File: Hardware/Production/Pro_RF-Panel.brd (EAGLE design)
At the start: 101.9 x 104.9 mm, 612 parts, among them U1 MCP73831, U10 915MHz, U11 ATMEGA32U4, U12 MIC5219-3.3, U13 MCP73831, U14 915MHz, U15 ATMEGA32U4, U16 MIC5219-3.3, U17 MCP73831, U18 915MHz, U19 ATMEGA32U4, U2 915MHz, U20 MIC5219-3.3, U21 MCP73831, U22 915MHz, U23 ATMEGA32U4, U24 MIC5219-3.3, U3 MCP73831, U4 915MHz, U5 ATMEGA32U4, U6 MIC5219-3.3, U7 ATMEGA32U4, U8 MIC5219-3.3, U9 MCP73831, Y1 8MHz, Y2 8MHz, Y3 8MHz, Y4 8MHz, Y5 8MHz, Y6 8MHz

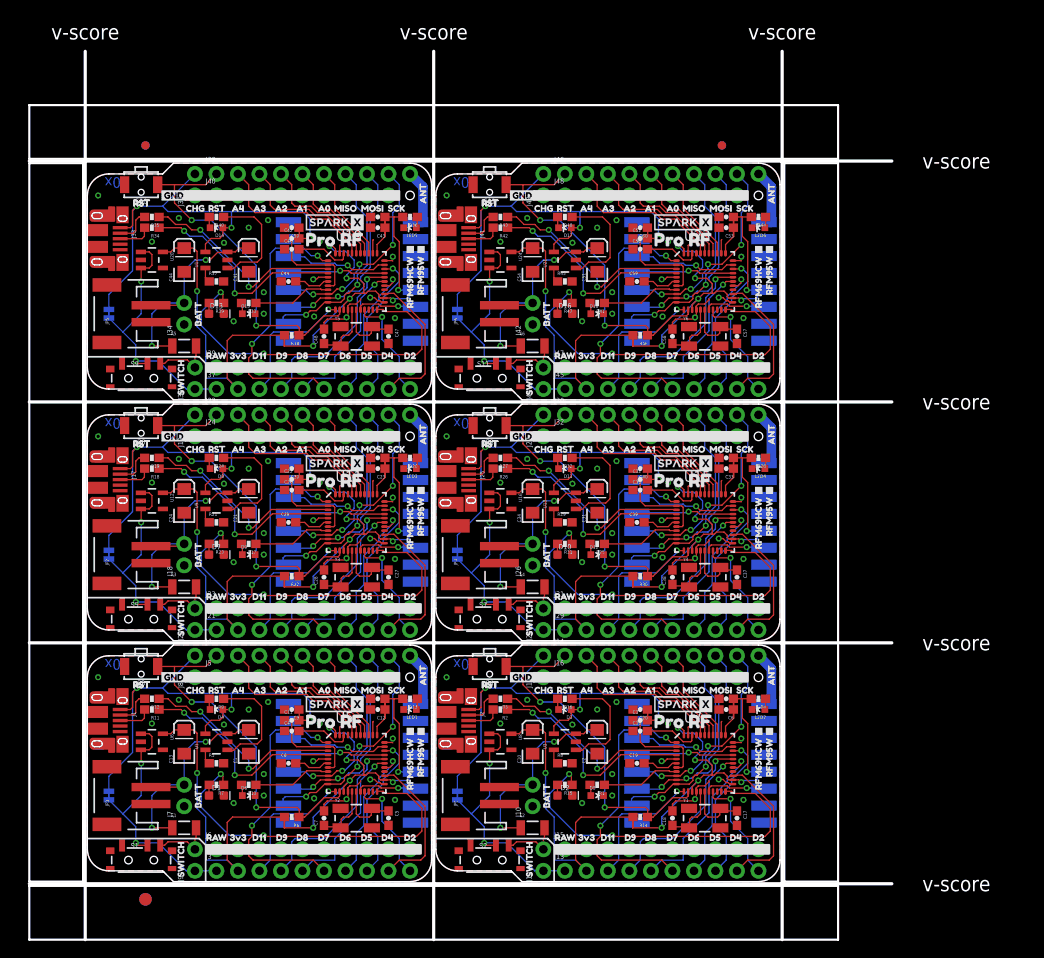
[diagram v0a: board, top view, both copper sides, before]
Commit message: Many updates. v02.
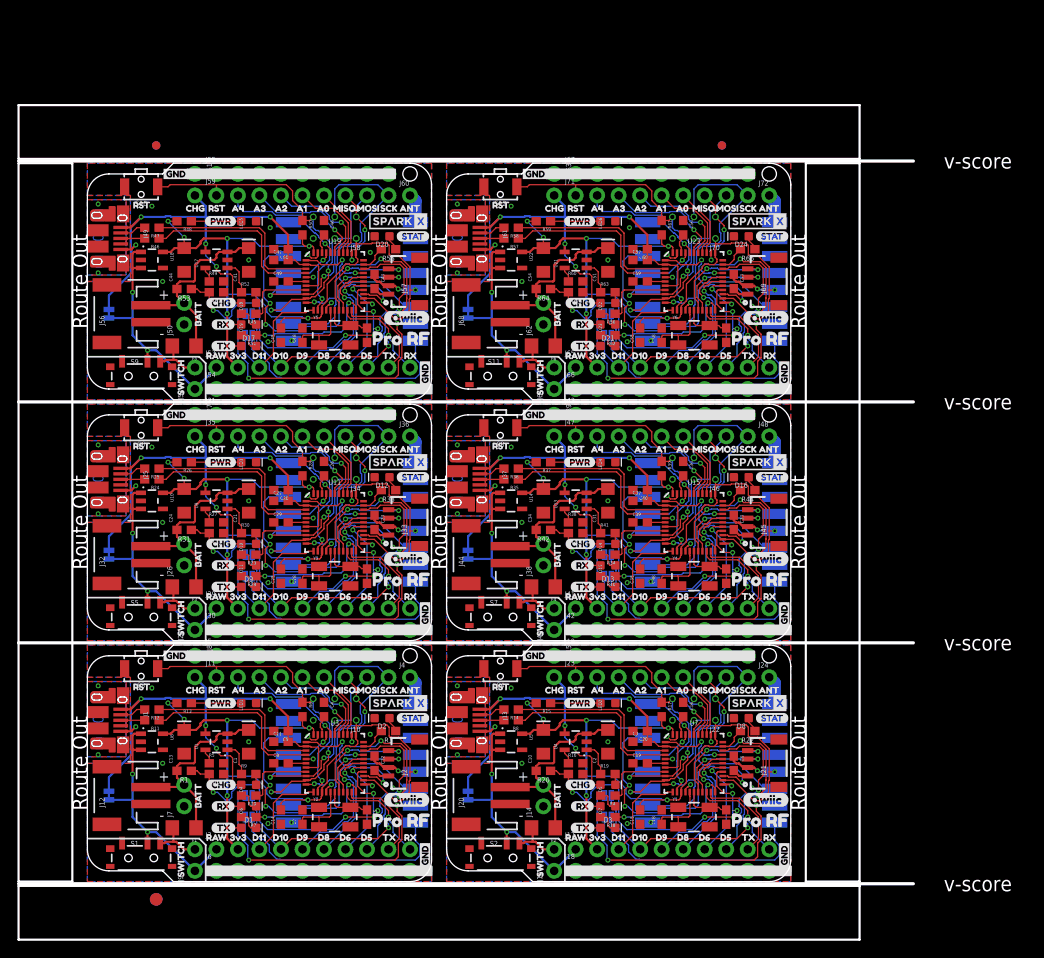
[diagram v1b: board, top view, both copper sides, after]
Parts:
- added D19, D22, D23: Yellow, SparkFun-LED:LED-0603
- added D20, D24: BLUE, SparkFun-LED:LED-0603
- added D21: Green, SparkFun-LED:LED-0603
- added J49, J61: (no value), SparkFun-Connectors:USB-MICROB-PTH-MILL
- added J50, J62: PTH, SparkFun-Connectors:1X02_NO_SILK
- added J51, J63: (no value), SparkFun-Connectors:1X02_NO_SILK
- added J52, J64: External On/Off, SparkFun-Connectors:1X02_NO_SILK
- added J53, J54, J65, J66: (no value), SparkFun-Connectors:1X10_NO_SILK
- added J55, J59, J67, J71: (no value), SparkFun-Connectors:1X09_NO_SILK
- added J56, J68: JST, SparkFun-Connectors:JST-2-SMD
- added J57, J69: (no value), SparkFun-Connectors:1X04_1MM_RA
- added J58, J70: AVR_SPI_PROG_3X2TESTPOINTS, SparkFun-Connectors:2X3_TEST_POINTS
- added J60, J72: (no value), SparkFun-Connectors:1X01_NO_SILK
- added JP10, JP11, JP12, JP7, JP8, JP9: (no value), SparkFun-Jumpers:SMT-JUMPER_2_NO_SILK
- added R49, R60: 2.0k, SparkFun-Resistors:0603
- added R50, R53, R54, R61, R64, R65: 10k, SparkFun-Resistors:0603
- added R51, R52, R55, R56, R59, R62, R63, R66: 1k, SparkFun-Resistors:0603
- added R57, R58: 22, SparkFun-Resistors:0603
- added U$367, U$396: (no value), buzzard_labels (25):D1119
- added U$368, U$395: (no value), buzzard_labels (25):3V320
- added U$369, U$394: (no value), buzzard_labels (25):RAW21
- added U$370, U$379: (no value), buzzard_labels (25):SWITCH23
- added U$371, U$378, U$383: (no value), buzzard_labels (25):RST2
- added U$372, U$375: (no value), buzzard_labels (25):BATT25
- added U$373: (no value), SparkX:SPARKX-SMALL
- added U$374: (no value), buzzard_labels (24):PRO_RF0
- added U$376: (no value), buzzard_labels (27):CUT_IF_RAW_IN0
- added U$377: (no value), buzzard_labels (27):GREATER_THAN_5#5V1
- added U$380, U$399, U$414: (no value), buzzard_labels (25):GND0
- added U$381: (no value), buzzard_labels (28):ON#OFF0
- added U$382: (no value), buzzard_labels (25):CHG1
- added U$384: (no value), buzzard_labels (25):A43
- added U$385: (no value), buzzard_labels (25):A34
- added U$386: (no value), buzzard_labels (25):A25
- added U$387: (no value), buzzard_labels (25):A16
- added U$388: (no value), buzzard_labels (25):A07
- added U$389: (no value), buzzard_labels (25):MISO8
- added U$390: (no value), buzzard_labels (25):MOSI9
- added U$391: (no value), buzzard_labels (25):SCK10
- added U$392: (no value), buzzard_labels (25):ANT11
- added U$393: (no value), SparkFun-Aesthetics:OSHW-LOGO-S
- added U$397: (no value), buzzard_labels (25):D817
- added U$398: (no value), buzzard_labels (25):D615
- added U$400: (no value), Labels:PWR-()-03
- added U$401: (no value), Labels:QWIIC-()-04
- added U$402, U$416: (no value), buzzard_labels (8):TX3
- added U$403: (no value), buzzard_labels (8):TX6
- added U$404: (no value), buzzard_labels (8):STAT5
- added U$405: (no value), buzzard_labels (8):RX7
- added U$406, U$415: (no value), buzzard_labels (8):RX2
- added U$407: (no value), buzzard_labels (9):CHG1
- added U$408, U$409: (no value), buzzard_labels (9):D100
- added U$410, U$411: (no value), buzzard_labels (25):D514
- added U$412, U$413: (no value), buzzard_labels (10):D90
- added U$417: (no value), buzzard_labels (12):RFM69HCW#1
- added U$418: (no value), buzzard_labels (12):RFM95W#0
- added U$419: (no value), buzzard_labels (3):LORA0
- added U$420: (no value), buzzard_labels (3):WAN1
- C1, C10, C13, C2, C21, C24, C31, C34, C41, C44, C51, C54: device SparkFun:EIA3216 -> SparkFun-Capacitors:EIA3216
- C11, C22, C3, C32, C42, C52: value 1uF -> 0.1uF; device SparkFun-Capacitors:0603-CAP -> SparkFun-Capacitors:0603
- C12, C19, C23, C29, C33, C39, C43, C49, C53, C59, C6, C8: value 1uF -> 1.0uF; device SparkFun-Capacitors:0603-CAP -> SparkFun-Capacitors:0603
- C14, C15, C16, C17, C18, C20, C25, C26, C27, C28, C30, C35, C36, C37, C38, C4, C40, C45, C46, C47, C48, C5, C50, C55, C56, C57, C58, C60, C7, C9: device SparkFun-Capacitors:0603-CAP -> SparkFun-Capacitors:0603
- D1, D13: value GREEN -> Green
- D10, D7: value GREEN -> Yellow
- D11, D14, D4: device SparkFun:LED-0603 -> SparkFun-LED:LED-0603
- D12: value Blue -> BLUE; device SparkFun:LED-0603 -> SparkFun-LED:LED-0603
- D15, D18, D5, D6: value Blue -> Yellow; device SparkFun:LED-0603 -> SparkFun-LED:LED-0603
- D16, D2: value GREEN -> BLUE
- D17, D3: value Yellow -> Green; device SparkFun:LED-0603 -> SparkFun-LED:LED-0603
- D8: value Yellow -> BLUE; device SparkFun:LED-0603 -> SparkFun-LED:LED-0603
- D9: value Blue -> Green; device SparkFun:LED-0603 -> SparkFun-LED:LED-0603
- F1, F2, F3, F4, F5, F6: value PTCSMD -> 6V/0.5A; device SparkFun:PTC-1206 -> SparkFun-Fuses:1206
- J10, J34: value (none) -> AVR_SPI_PROG_3X2TESTPOINTS; device SparkFun-Connectors:1X02_NO_SILK -> SparkFun-Connectors:2X3_TEST_POINTS
- J11, J19, J35, J43: device SparkFun-Connectors:1X02_NO_SILK -> SparkFun-Connectors:1X09_NO_SILK
- J12, J20, J44: value (none) -> JST; device SparkFun-Connectors:1X02_NO_SILK -> SparkFun-Connectors:JST-2-SMD
- J13, J37: device SparkFun-Connectors:1X10_NO_SILK -> SparkFun-Connectors:USB-MICROB-PTH-MILL
- J14, J38: value (none) -> PTH; device SparkFun-Connectors:1X10_NO_SILK -> SparkFun-Connectors:1X02_NO_SILK
- J15, J39: device SparkFun-Connectors:1X10_NO_SILK -> SparkFun-Connectors:1X02_NO_SILK
- J16, J40: value (none) -> External On/Off; device SparkFun-Connectors:1X09_NO_SILK -> SparkFun-Connectors:1X02_NO_SILK
- J17, J41: device SparkFun-Connectors:USB-MICROB-PTH-MILL -> SparkFun-Connectors:1X10_NO_SILK
- J18, J42: device SparkFun-Connectors:1X02_NO_SILK -> SparkFun-Connectors:1X10_NO_SILK
- J2, J33: device SparkFun-Connectors:USB-MICROB-PTH-MILL -> SparkFun-Connectors:1X04_1MM_RA
- J21, J45: device SparkFun-Connectors:1X10_NO_SILK -> SparkFun-Connectors:1X04_1MM_RA
- J22, J46: value (none) -> AVR_SPI_PROG_3X2TESTPOINTS; device SparkFun-Connectors:1X10_NO_SILK -> SparkFun-Connectors:2X3_TEST_POINTS
- J23, J31, J47: device SparkFun-Connectors:1X10_NO_SILK -> SparkFun-Connectors:1X09_NO_SILK
- J24, J48: device SparkFun-Connectors:1X09_NO_SILK -> SparkFun-Connectors:1X01_NO_SILK
- J26, J7: value (none) -> PTH
- J28, J9: value (none) -> External On/Off
- J32: value (none) -> JST; device SparkFun-Connectors:1X09_NO_SILK -> SparkFun-Connectors:JST-2-SMD
- J36: device SparkFun-Connectors:1X02_NO_SILK -> SparkFun-Connectors:1X01_NO_SILK
- J4: device SparkFun-Connectors:1X10_NO_SILK -> SparkFun-Connectors:1X01_NO_SILK
- JP1, JP2, JP3, JP4, JP5, JP6: device SparkFun:JST-2-SMD -> SparkFun-Jumpers:SMT-JUMPER_2_NO_SILK
- LED1, LED2, LED3, LED4, LED5, LED6: value Red -> RED; device SparkFun:LED-0603 -> SparkFun-LED:LED-0603
- R1, R17, R20, R28, R31, R39: value 330 -> 10k; device SparkFun-Resistors:0603-RES -> SparkFun-Resistors:0603
- R10, R13, R15, R23, R33, R4, R41, R44, R7: value 330 -> 1k; device SparkFun-Resistors:0603-RES -> SparkFun-Resistors:0603
- R11, R12, R35: device SparkFun-Resistors:0603-RES -> SparkFun-Resistors:0603
- R14, R46: value 10K -> 22; device SparkFun-Resistors:0603-RES -> SparkFun-Resistors:0603
- R16: value 470 -> 2.0k; device SparkFun-Resistors:0603-RES -> SparkFun-Resistors:0603
- R18, R19, R26, R3, R34: value 22 -> 1k; device SparkFun-Resistors:0603-RES -> SparkFun-Resistors:0603
- R2, R42, R43: value 22 -> 10k; device SparkFun-Resistors:0603-RES -> SparkFun-Resistors:0603
- R21: value 2K -> 10k; device SparkFun-Resistors:0603-RES -> SparkFun-Resistors:0603
- R22, R30: value 10K -> 1k; device SparkFun-Resistors:0603-RES -> SparkFun-Resistors:0603
- R24: value 470 -> 22; device SparkFun-Resistors:0603-RES -> SparkFun-Resistors:0603
- R25, R36, R47: value 330 -> 22; device SparkFun-Resistors:0603-RES -> SparkFun-Resistors:0603
- R27: value 22 -> 2.0k; device SparkFun-Resistors:0603-RES -> SparkFun-Resistors:0603
- R29, R37, R45: value 2K -> 1k; device SparkFun-Resistors:0603-RES -> SparkFun-Resistors:0603
- R32: value 470 -> 10k; device SparkFun-Resistors:0603-RES -> SparkFun-Resistors:0603
- R38: value 10K -> 2.0k; device SparkFun-Resistors:0603-RES -> SparkFun-Resistors:0603
- R40, R48, R9: value 470 -> 1k; device SparkFun-Resistors:0603-RES -> SparkFun-Resistors:0603
- R5: value 2K -> 2.0k; device SparkFun-Resistors:0603-RES -> SparkFun-Resistors:0603
- R6: value 10K -> 10k; device SparkFun-Resistors:0603-RES -> SparkFun-Resistors:0603
- R8: value 2K -> 22; device SparkFun-Resistors:0603-RES -> SparkFun-Resistors:0603
- S1, S11, S2, S5, S7, S9: value (none) -> Power
- S10, S12, S3, S4, S6, S8: value MOMENTARY-SWITCH-SPST-SMD-RIGHT-ANGLE -> (none)
- SJ1, SJ2, SJ3, SJ4, SJ5, SJ6: device SparkFun:SJ_2S-TRACE -> SparkFun-Jumpers:SMT-JUMPER_2_NC_TRACE_SILK
- U$100, U$222, U$344: device buzzard_labels (28):ON#OFF0 -> buzzard_labels (25):GND0
- U$101: device buzzard_labels (25):CHG1 -> buzzard_labels (28):ON#OFF0
- U$102, U$224: device buzzard_labels (25):RST2 -> buzzard_labels (25):CHG1
- U$103, U$308: device buzzard_labels (25):A43 -> buzzard_labels (25):RST2
- U$104: device buzzard_labels (25):A34 -> buzzard_labels (25):A43
- U$105: device buzzard_labels (25):A25 -> buzzard_labels (25):A34
- U$106: device buzzard_labels (25):A16 -> buzzard_labels (25):A25
- U$107: device buzzard_labels (25):A07 -> buzzard_labels (25):A16
- U$108: device buzzard_labels (25):MISO8 -> buzzard_labels (25):A07
- U$109: device buzzard_labels (25):MOSI9 -> buzzard_labels (25):MISO8
- U$110: device buzzard_labels (25):SCK10 -> buzzard_labels (25):MOSI9
- U$111: device buzzard_labels (25):ANT11 -> buzzard_labels (25):SCK10
- U$112: device SparkFun-Aesthetics:OSHW-LOGO-S -> buzzard_labels (25):ANT11
- U$113: device buzzard_labels (25):RAW21 -> SparkFun-Aesthetics:OSHW-LOGO-S
- U$114: device buzzard_labels (25):3V320 -> buzzard_labels (25):RAW21
- U$115, U$298: device buzzard_labels (25):D1119 -> buzzard_labels (25):3V320
- U$116, U$326: device buzzard_labels (25):D918 -> buzzard_labels (25):D1119
- U$118: device buzzard_labels (25):D716 -> buzzard_labels (25):D615
- U$119: device buzzard_labels (25):D615 -> buzzard_labels (25):GND0
- U$120: device buzzard_labels (25):D514 -> Labels:PWR-()-03
- U$121: device buzzard_labels (25):D413 -> Labels:QWIIC-()-04
- U$122: device buzzard_labels (25):D212 -> buzzard_labels (8):TX3
- U$123: device buzzard_labels (24):PRO_RF0 -> buzzard_labels (8):TX6
- U$124: device SparkX:SPARKX-SMALL -> buzzard_labels (8):STAT5
- U$125: device buzzard_labels (25):A43 -> buzzard_labels (8):RX7
- U$126: device buzzard_labels (25):A34 -> buzzard_labels (8):RX2
- U$127: device buzzard_labels (25):A25 -> buzzard_labels (9):CHG1
- U$128: device buzzard_labels (25):A16 -> buzzard_labels (9):D100
- U$129, U$68: device buzzard_labels (25):A07 -> buzzard_labels (9):D100
- U$130: device buzzard_labels (25):MISO8 -> buzzard_labels (25):D514
- U$131: device buzzard_labels (25):MOSI9 -> buzzard_labels (25):D514
- U$132: device buzzard_labels (25):SCK10 -> buzzard_labels (10):D90
- U$133: device buzzard_labels (25):ANT11 -> buzzard_labels (10):D90
- U$135, U$196: device buzzard_labels (25):RST2 -> buzzard_labels (8):RX2
- U$136: device buzzard_labels (25):CHG1 -> buzzard_labels (8):TX3
- U$137: device buzzard_labels (25):D212 -> buzzard_labels (12):RFM69HCW#1
- U$138, U$60: device buzzard_labels (25):D413 -> buzzard_labels (12):RFM95W#0
- U$139: device buzzard_labels (25):D514 -> buzzard_labels (3):LORA0
- U$140: device buzzard_labels (25):D615 -> buzzard_labels (3):WAN1
- U$141: device buzzard_labels (25):D716 -> buzzard_labels (24):PRO_RF0
- U$142: device buzzard_labels (25):D817 -> SparkX:SPARKX-SMALL
- U$143: device buzzard_labels (25):D918 -> buzzard_labels (25):A43
- U$144: device buzzard_labels (25):D1119 -> buzzard_labels (25):A34
- U$145: device buzzard_labels (25):3V320 -> buzzard_labels (25):A25
- U$146: device buzzard_labels (25):RAW21 -> buzzard_labels (25):A16
- U$147: device buzzard_labels (26):RFM69HCW_#0 -> buzzard_labels (25):A07
- U$148: device buzzard_labels (26):RFM95W_#1 -> buzzard_labels (25):MISO8
- U$149: device buzzard_labels (25):SWITCH23 -> buzzard_labels (25):MOSI9
- U$15: device buzzard_labels (25):D212 -> buzzard_labels (10):D90
- U$150: device buzzard_labels (25):RST2 -> buzzard_labels (25):SCK10
- U$151: device buzzard_labels (25):BATT25 -> buzzard_labels (25):ANT11
- U$152, U$274: device SparkX:SPARKX-SMALL -> buzzard_labels (25):GND0
- U$153: device buzzard_labels (24):PRO_RF0 -> buzzard_labels (25):RST2
- U$154: device buzzard_labels (25):BATT25 -> buzzard_labels (25):CHG1
- U$155: device buzzard_labels (27):CUT_IF_RAW_IN0 -> buzzard_labels (25):D615
- U$156: device buzzard_labels (27):GREATER_THAN_5#5V1 -> buzzard_labels (25):D817
- U$157: device buzzard_labels (25):RST2 -> buzzard_labels (25):D1119
- U$158: device buzzard_labels (25):RST2 -> buzzard_labels (25):3V320
- U$159: device buzzard_labels (25):SWITCH23 -> buzzard_labels (25):RAW21
- U$16: device buzzard_labels (25):D413 -> buzzard_labels (10):D90
- U$160, U$99: device buzzard_labels (25):GND0 -> buzzard_labels (25):SWITCH23
- U$161: device buzzard_labels (28):ON#OFF0 -> buzzard_labels (25):RST2
- U$162: device buzzard_labels (25):CHG1 -> buzzard_labels (25):BATT25
- U$163: device buzzard_labels (25):RST2 -> SparkX:SPARKX-SMALL
- U$164: device buzzard_labels (25):A43 -> buzzard_labels (24):PRO_RF0
- U$165: device buzzard_labels (25):A34 -> buzzard_labels (25):BATT25
- U$166: device buzzard_labels (25):A25 -> buzzard_labels (27):CUT_IF_RAW_IN0
- U$167: device buzzard_labels (25):A16 -> buzzard_labels (27):GREATER_THAN_5#5V1
- U$168: device buzzard_labels (25):A07 -> buzzard_labels (25):RST2
- U$169, U$230: device buzzard_labels (25):MISO8 -> buzzard_labels (25):SWITCH23
- U$17: device buzzard_labels (25):D514 -> buzzard_labels (25):GND0
- U$170, U$292: device buzzard_labels (25):MOSI9 -> buzzard_labels (25):GND0
- U$171: device buzzard_labels (25):SCK10 -> buzzard_labels (28):ON#OFF0
- U$172, U$294: device buzzard_labels (25):ANT11 -> buzzard_labels (25):CHG1
- U$173: device SparkFun-Aesthetics:OSHW-LOGO-S -> buzzard_labels (25):RST2
- U$174: device buzzard_labels (25):RAW21 -> buzzard_labels (25):A43
- U$175: device buzzard_labels (25):3V320 -> buzzard_labels (25):A34
- U$176: device buzzard_labels (25):D1119 -> buzzard_labels (25):A25
- U$177: device buzzard_labels (25):D918 -> buzzard_labels (25):A16
- U$178: device buzzard_labels (25):D817 -> buzzard_labels (25):A07
- U$179: device buzzard_labels (25):D716 -> buzzard_labels (25):MISO8
- U$180, U$79: device buzzard_labels (25):D615 -> buzzard_labels (25):MOSI9
- U$181: device buzzard_labels (25):D514 -> buzzard_labels (25):SCK10
- U$182: device buzzard_labels (25):D413 -> buzzard_labels (25):ANT11
- U$183: device buzzard_labels (25):D212 -> SparkFun-Aesthetics:OSHW-LOGO-S
- U$184: device buzzard_labels (24):PRO_RF0 -> buzzard_labels (25):RAW21
- U$185: device SparkX:SPARKX-SMALL -> buzzard_labels (25):3V320
- U$186: device buzzard_labels (25):A43 -> buzzard_labels (25):D1119
- U$187, U$226: device buzzard_labels (25):A34 -> buzzard_labels (25):D817
- U$188: device buzzard_labels (25):A25 -> buzzard_labels (25):D615
- U$189: device buzzard_labels (25):A16 -> buzzard_labels (25):GND0
- U$19: device buzzard_labels (25):D716 -> buzzard_labels (8):RX2
- U$190: device buzzard_labels (25):A07 -> Labels:PWR-()-03
- U$191: device buzzard_labels (25):MISO8 -> Labels:QWIIC-()-04
- U$192: device buzzard_labels (25):MOSI9 -> buzzard_labels (8):TX3
- U$193: device buzzard_labels (25):SCK10 -> buzzard_labels (8):TX6
- U$194: device buzzard_labels (25):ANT11 -> buzzard_labels (8):STAT5
- U$195: device buzzard_labels (25):GND0 -> buzzard_labels (8):RX7
- U$197: device buzzard_labels (25):CHG1 -> buzzard_labels (9):CHG1
- U$198: device buzzard_labels (25):D212 -> buzzard_labels (9):D100
- U$199: device buzzard_labels (25):D413 -> buzzard_labels (9):D100
- U$201: device buzzard_labels (25):D615 -> buzzard_labels (25):D514
- U$202: device buzzard_labels (25):D716 -> buzzard_labels (10):D90
- U$203: device buzzard_labels (25):D817 -> buzzard_labels (10):D90
- U$204, U$82: device buzzard_labels (25):D918 -> buzzard_labels (25):GND0
- U$205, U$266: device buzzard_labels (25):D1119 -> buzzard_labels (8):RX2
- U$206: device buzzard_labels (25):3V320 -> buzzard_labels (8):TX3
- U$207: device buzzard_labels (25):RAW21 -> buzzard_labels (12):RFM69HCW#1
- U$208: device buzzard_labels (26):RFM69HCW_#0 -> buzzard_labels (12):RFM95W#0
- U$209: device buzzard_labels (26):RFM95W_#1 -> buzzard_labels (3):LORA0
- U$21: device buzzard_labels (25):D918 -> buzzard_labels (9):D100
- U$210: device buzzard_labels (25):SWITCH23 -> buzzard_labels (3):WAN1
- U$211: device buzzard_labels (25):RST2 -> buzzard_labels (24):PRO_RF0
- U$212, U$93: device buzzard_labels (25):BATT25 -> SparkX:SPARKX-SMALL
- U$213: device SparkX:SPARKX-SMALL -> buzzard_labels (25):A43
- U$214, U$245: device buzzard_labels (24):PRO_RF0 -> buzzard_labels (25):A34
- U$215: device buzzard_labels (25):BATT25 -> buzzard_labels (25):A25
- U$216: device buzzard_labels (27):CUT_IF_RAW_IN0 -> buzzard_labels (25):A16
- U$217: device buzzard_labels (27):GREATER_THAN_5#5V1 -> buzzard_labels (25):A07
- U$218: device buzzard_labels (25):RST2 -> buzzard_labels (25):MISO8
- U$219: device buzzard_labels (25):RST2 -> buzzard_labels (25):MOSI9
- U$220: device buzzard_labels (25):SWITCH23 -> buzzard_labels (25):SCK10
- U$221: device buzzard_labels (25):GND0 -> buzzard_labels (25):ANT11
- U$223: device buzzard_labels (25):CHG1 -> buzzard_labels (25):RST2
- U$225: device buzzard_labels (25):A43 -> buzzard_labels (25):D615
- U$227: device buzzard_labels (25):A25 -> buzzard_labels (25):D1119
- U$228: device buzzard_labels (25):A16 -> buzzard_labels (25):3V320
- U$229: device buzzard_labels (25):A07 -> buzzard_labels (25):RAW21
- U$231: device buzzard_labels (25):MOSI9 -> buzzard_labels (25):RST2
- U$232: device buzzard_labels (25):SCK10 -> buzzard_labels (25):BATT25
- U$233: device buzzard_labels (25):ANT11 -> SparkX:SPARKX-SMALL
- U$234: device SparkFun-Aesthetics:OSHW-LOGO-S -> buzzard_labels (24):PRO_RF0
- U$235: device buzzard_labels (25):RAW21 -> buzzard_labels (25):BATT25
- U$236: device buzzard_labels (25):3V320 -> buzzard_labels (27):CUT_IF_RAW_IN0
- U$237: device buzzard_labels (25):D1119 -> buzzard_labels (27):GREATER_THAN_5#5V1
- U$238: device buzzard_labels (25):D918 -> buzzard_labels (25):RST2
- U$239, U$300: device buzzard_labels (25):D817 -> buzzard_labels (25):SWITCH23
- U$240, U$362: device buzzard_labels (25):D716 -> buzzard_labels (25):GND0
- U$241: device buzzard_labels (25):D615 -> buzzard_labels (28):ON#OFF0
- U$242, U$364: device buzzard_labels (25):D514 -> buzzard_labels (25):CHG1
- U$243: device buzzard_labels (25):D413 -> buzzard_labels (25):RST2
- U$244: device buzzard_labels (25):D212 -> buzzard_labels (25):A43
- U$246: device SparkX:SPARKX-SMALL -> buzzard_labels (25):A25
- U$247, U$286: device buzzard_labels (25):A43 -> buzzard_labels (25):A16
- U$248, U$287: device buzzard_labels (25):A34 -> buzzard_labels (25):A07
- U$249, U$288: device buzzard_labels (25):A25 -> buzzard_labels (25):MISO8
- U$25: device buzzard_labels (26):RFM69HCW_#0 -> buzzard_labels (3):LORA0
- U$250, U$289: device buzzard_labels (25):A16 -> buzzard_labels (25):MOSI9
- U$251, U$290: device buzzard_labels (25):A07 -> buzzard_labels (25):SCK10
- U$252, U$291: device buzzard_labels (25):MISO8 -> buzzard_labels (25):ANT11
- U$253: device buzzard_labels (25):MOSI9 -> SparkFun-Aesthetics:OSHW-LOGO-S
- U$254: device buzzard_labels (25):SCK10 -> buzzard_labels (25):RAW21
- U$255: device buzzard_labels (25):ANT11 -> buzzard_labels (25):3V320
- U$256: device buzzard_labels (25):GND0 -> buzzard_labels (25):D1119
- U$257: device buzzard_labels (25):RST2 -> buzzard_labels (25):D817
- U$258: device buzzard_labels (25):CHG1 -> buzzard_labels (25):D615
- U$259: device buzzard_labels (25):D212 -> buzzard_labels (25):GND0
- U$26: device buzzard_labels (26):RFM95W_#1 -> buzzard_labels (24):PRO_RF0
- U$260: device buzzard_labels (25):D413 -> Labels:PWR-()-03
- U$261: device buzzard_labels (25):D514 -> Labels:QWIIC-()-04
- U$262: device buzzard_labels (25):D615 -> buzzard_labels (8):TX3
- U$263: device buzzard_labels (25):D716 -> buzzard_labels (8):TX6
- U$264: device buzzard_labels (25):D817 -> buzzard_labels (8):STAT5
- U$265: device buzzard_labels (25):D918 -> buzzard_labels (8):RX7
- U$267: device buzzard_labels (25):3V320 -> buzzard_labels (9):CHG1
- U$268: device buzzard_labels (25):RAW21 -> buzzard_labels (9):D100
- U$269: device buzzard_labels (26):RFM69HCW_#0 -> buzzard_labels (9):D100
- U$270: device buzzard_labels (26):RFM95W_#1 -> buzzard_labels (25):D514
- U$271: device buzzard_labels (25):SWITCH23 -> buzzard_labels (25):D514
- U$272: device buzzard_labels (25):RST2 -> buzzard_labels (10):D90
- U$273: device buzzard_labels (25):BATT25 -> buzzard_labels (10):D90
- U$275, U$336: device buzzard_labels (24):PRO_RF0 -> buzzard_labels (8):RX2
- U$276: device buzzard_labels (25):BATT25 -> buzzard_labels (8):TX3
- U$277: device buzzard_labels (27):CUT_IF_RAW_IN0 -> buzzard_labels (12):RFM69HCW#1
- U$278: device buzzard_labels (27):GREATER_THAN_5#5V1 -> buzzard_labels (12):RFM95W#0
- U$279: device buzzard_labels (25):RST2 -> buzzard_labels (3):LORA0
- U$280, U$35: device buzzard_labels (25):RST2 -> buzzard_labels (3):WAN1
- U$281: device buzzard_labels (25):SWITCH23 -> buzzard_labels (24):PRO_RF0
- U$282: device buzzard_labels (25):GND0 -> SparkX:SPARKX-SMALL
- U$283: device buzzard_labels (28):ON#OFF0 -> buzzard_labels (25):A43
- U$284: device buzzard_labels (25):CHG1 -> buzzard_labels (25):A34
- U$285: device buzzard_labels (25):RST2 -> buzzard_labels (25):A25
- U$293: device buzzard_labels (25):SCK10 -> buzzard_labels (25):RST2
- U$295: device SparkFun-Aesthetics:OSHW-LOGO-S -> buzzard_labels (25):D615
- U$296: device buzzard_labels (25):RAW21 -> buzzard_labels (25):D817
- U$297: device buzzard_labels (25):3V320 -> buzzard_labels (25):D1119
- U$299: device buzzard_labels (25):D918 -> buzzard_labels (25):RAW21
- U$301: device buzzard_labels (25):D716 -> buzzard_labels (25):RST2
- U$302: device buzzard_labels (25):D615 -> buzzard_labels (25):BATT25
- U$303: device buzzard_labels (25):D514 -> SparkX:SPARKX-SMALL
- U$304: device buzzard_labels (25):D413 -> buzzard_labels (24):PRO_RF0
- U$305: device buzzard_labels (25):D212 -> buzzard_labels (25):BATT25
- U$306: device buzzard_labels (24):PRO_RF0 -> buzzard_labels (27):CUT_IF_RAW_IN0
- U$307: device SparkX:SPARKX-SMALL -> buzzard_labels (27):GREATER_THAN_5#5V1
- U$309: device buzzard_labels (25):A34 -> buzzard_labels (25):SWITCH23
- U$310: device buzzard_labels (25):A25 -> buzzard_labels (25):GND0
- U$311: device buzzard_labels (25):A16 -> buzzard_labels (28):ON#OFF0
- U$312: device buzzard_labels (25):A07 -> buzzard_labels (25):CHG1
- U$313: device buzzard_labels (25):MISO8 -> buzzard_labels (25):RST2
- U$314, U$353: device buzzard_labels (25):MOSI9 -> buzzard_labels (25):A43
- U$315, U$354: device buzzard_labels (25):SCK10 -> buzzard_labels (25):A34
- U$316, U$355: device buzzard_labels (25):ANT11 -> buzzard_labels (25):A25
- U$317: device buzzard_labels (25):GND0 -> buzzard_labels (25):A16
- U$318: device buzzard_labels (25):RST2 -> buzzard_labels (25):A07
- U$319: device buzzard_labels (25):CHG1 -> buzzard_labels (25):MISO8
- U$320: device buzzard_labels (25):D212 -> buzzard_labels (25):MOSI9
- U$321: device buzzard_labels (25):D413 -> buzzard_labels (25):SCK10
- U$322: device buzzard_labels (25):D514 -> buzzard_labels (25):ANT11
- U$323: device buzzard_labels (25):D615 -> SparkFun-Aesthetics:OSHW-LOGO-S
- U$324: device buzzard_labels (25):D716 -> buzzard_labels (25):RAW21
- U$325: device buzzard_labels (25):D817 -> buzzard_labels (25):3V320
- U$327: device buzzard_labels (25):D1119 -> buzzard_labels (25):D817
- U$328: device buzzard_labels (25):3V320 -> buzzard_labels (25):D615
- U$329: device buzzard_labels (25):RAW21 -> buzzard_labels (25):GND0
- U$330: device buzzard_labels (26):RFM69HCW_#0 -> Labels:PWR-()-03
- U$331: device buzzard_labels (26):RFM95W_#1 -> Labels:QWIIC-()-04
- U$332: device buzzard_labels (25):SWITCH23 -> buzzard_labels (8):TX3
- U$333: device buzzard_labels (25):RST2 -> buzzard_labels (8):TX6
- U$334: device buzzard_labels (25):BATT25 -> buzzard_labels (8):STAT5
- U$335: device SparkX:SPARKX-SMALL -> buzzard_labels (8):RX7
- U$337: device buzzard_labels (25):BATT25 -> buzzard_labels (9):CHG1
- U$338: device buzzard_labels (27):CUT_IF_RAW_IN0 -> buzzard_labels (9):D100
- U$339: device buzzard_labels (27):GREATER_THAN_5#5V1 -> buzzard_labels (9):D100
- U$340, U$341, U$74: device buzzard_labels (25):RST2 -> buzzard_labels (25):D514
- U$342: device buzzard_labels (25):SWITCH23 -> buzzard_labels (10):D90
- U$343: device buzzard_labels (25):GND0 -> buzzard_labels (10):D90
- U$345: device buzzard_labels (25):CHG1 -> buzzard_labels (8):RX2
- U$346: device buzzard_labels (25):RST2 -> buzzard_labels (8):TX3
- U$347: device buzzard_labels (25):A43 -> buzzard_labels (12):RFM69HCW#1
- U$348: device buzzard_labels (25):A34 -> buzzard_labels (12):RFM95W#0
- U$349: device buzzard_labels (25):A25 -> buzzard_labels (3):LORA0
- U$350: device buzzard_labels (25):A16 -> buzzard_labels (3):WAN1
- U$351: device buzzard_labels (25):A07 -> buzzard_labels (24):PRO_RF0
- U$352: device buzzard_labels (25):MISO8 -> SparkX:SPARKX-SMALL
- U$356: device SparkFun-Aesthetics:OSHW-LOGO-S -> buzzard_labels (25):A16
- U$357: device buzzard_labels (25):RAW21 -> buzzard_labels (25):A07
- U$358: device buzzard_labels (25):3V320 -> buzzard_labels (25):MISO8
- U$359: device buzzard_labels (25):D1119 -> buzzard_labels (25):MOSI9
- U$360: device buzzard_labels (25):D918 -> buzzard_labels (25):SCK10
- U$361, U$81: device buzzard_labels (25):D817 -> buzzard_labels (25):ANT11
- U$363: device buzzard_labels (25):D615 -> buzzard_labels (25):RST2
- U$365: device buzzard_labels (25):D413 -> buzzard_labels (25):D615
- U$366: device buzzard_labels (25):D212 -> buzzard_labels (25):D817
- U$55: device buzzard_labels (25):D918 -> buzzard_labels (25):D514
- U$57: device buzzard_labels (25):D716 -> buzzard_labels (8):TX3
- U$59: device buzzard_labels (25):D514 -> buzzard_labels (12):RFM69HCW#1
- U$61: device buzzard_labels (25):D212 -> SparkX:SPARKX-SMALL
- U$62: device buzzard_labels (24):PRO_RF0 -> buzzard_labels (25):GND0
- U$63: device SparkX:SPARKX-SMALL -> Labels:PWR-()-03
- U$65: device buzzard_labels (25):A34 -> buzzard_labels (9):CHG1
- U$66: device buzzard_labels (25):A25 -> Labels:QWIIC-()-04
- U$67: device buzzard_labels (25):A16 -> buzzard_labels (25):A34
- U$69: device buzzard_labels (25):MISO8 -> buzzard_labels (8):TX3
- U$70: device buzzard_labels (25):MOSI9 -> buzzard_labels (8):TX6
- U$71: device buzzard_labels (25):SCK10 -> buzzard_labels (8):STAT5
- U$72: device buzzard_labels (25):ANT11 -> buzzard_labels (8):RX7
- U$73: device buzzard_labels (25):GND0 -> buzzard_labels (8):RX2
- U$75: device buzzard_labels (25):CHG1 -> buzzard_labels (25):A25
- U$76: device buzzard_labels (25):D212 -> buzzard_labels (25):A16
- U$77: device buzzard_labels (25):D413 -> buzzard_labels (25):A07
- U$78: device buzzard_labels (25):D514 -> buzzard_labels (25):MISO8
- U$80: device buzzard_labels (25):D716 -> buzzard_labels (25):SCK10
- U$83: device buzzard_labels (25):D1119 -> buzzard_labels (25):RST2
- U$84: device buzzard_labels (25):3V320 -> buzzard_labels (25):CHG1
- U$85: device buzzard_labels (25):RAW21 -> buzzard_labels (25):D615
- U$86: device buzzard_labels (26):RFM69HCW_#0 -> buzzard_labels (25):D817
- U$87: device buzzard_labels (26):RFM95W_#1 -> buzzard_labels (25):D1119
- U$88: device buzzard_labels (25):SWITCH23 -> buzzard_labels (25):3V320
- U$89: device buzzard_labels (25):RST2 -> buzzard_labels (25):RAW21
- U$90: device buzzard_labels (25):BATT25 -> buzzard_labels (25):SWITCH23
- U$91: device SparkX:SPARKX-SMALL -> buzzard_labels (25):RST2
- U$92: device buzzard_labels (24):PRO_RF0 -> buzzard_labels (25):BATT25
- U$94: device buzzard_labels (27):CUT_IF_RAW_IN0 -> buzzard_labels (24):PRO_RF0
- U$95: device buzzard_labels (27):GREATER_THAN_5#5V1 -> buzzard_labels (25):BATT25
- U$96: device buzzard_labels (25):RST2 -> buzzard_labels (27):CUT_IF_RAW_IN0
- U$97: device buzzard_labels (25):RST2 -> buzzard_labels (27):GREATER_THAN_5#5V1
- U$98: device buzzard_labels (25):SWITCH23 -> buzzard_labels (25):RST2
- U1, U13, U17, U21, U9: device SparkFun:SOT23-5 -> SparkFun-IC-Power:SOT23-5
- U10, U14, U18, U22: value 915MHz -> 3.3V; device SparkFun-RF:RFM69HCW-XXXS2 -> SparkFun-IC-Power:SOT23-5
- U11, U15, U19, U23, U7: value ATMEGA32U4 -> 32U4; device Testing:QFN-44-NOPAD_1:1 -> SparkFun-IC-Microcontroller:QFN-44-NOPAD
- U12, U16, U20, U24, U8: value MIC5219-3.3 -> 915MHz; device SparkFun:SOT23-5 -> SparkFun-RF:RFM69HCW-XXXS2
- U3: value MCP73831 -> 32U4; device SparkFun:SOT23-5 -> SparkFun-IC-Microcontroller:QFN-44-NOPAD
- U4: value 915MHz -> MCP73831; device SparkFun-RF:RFM69HCW-XXXS2 -> SparkFun-IC-Power:SOT23-5
- U5: value ATMEGA32U4 -> 3.3V; device Testing:QFN-44-NOPAD_1:1 -> SparkFun-IC-Power:SOT23-5
- U6: value MIC5219-3.3 -> 3.3V; device SparkFun:SOT23-5 -> SparkFun-IC-Power:SOT23-5
- Y1, Y2, Y3, Y4, Y5, Y6: device SparkFun:CRYSTAL-SMD-5X3 -> SparkFun-Clocks:CRYSTAL-SMD-5X3.2-4PAD
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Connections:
- removed net A30: J46.6, U23.36
- removed net A31: J46.5, U23.37
- removed net A32: J46.4, U23.38
- removed net A33: J46.3, U23.39
- removed net A34: J46.2, U23.40
- removed net A35: U23.41
- removed net D37: J29.8, U15.31
- removed net D38: J29.7, U15.27
- removed net D39: J29.5, U15.28
- removed net D40: U14.5, U15.30
- removed net D41: J29.6, U15.1
- removed net D42: J29.4, U15.29
- removed net D43: J29.3, U15.12
- removed net D44: R25.1, U15.8
- removed net D45: J37.10, U19.19
- removed net D46: U18.14, U19.18
- removed net D47: J37.9, U19.25
- removed net D48: J37.8, U19.31
- removed net D49: J37.7, U19.27
- removed net D50: J37.5, U19.28
- removed net D51: U18.5, U19.30
- removed net D52: J37.6, U19.1
- removed net D53: J37.4, U19.29
- removed net D54: J37.3, U19.12
- removed net D55: R33.1, U19.8
- removed net D56: J45.10, U23.19
- removed net D57: U22.14, U23.18
- removed net D58: J45.9, U23.25
- removed net D59: J45.8, U23.31
- removed net D60: J45.7, U23.27
- removed net D61: J45.5, U23.28
- removed net D62: U22.5, U23.30
- removed net D63: J45.6, U23.1
- removed net D64: J45.4, U23.29
- removed net D65: J45.3, U23.12
- removed net D66: R41.1, U23.8
- removed net N$23 (its old number): D9.A, R17.2
- removed net N$33 (its old number): D12.A, R25.2
- removed net N$34 (its old number): J25.D-, R27.2
- removed net N$4 (its old number): D5.A, R1.2
- removed net N$45 (its old number): J33.D-, R35.2
- removed net N$46 (its old number): J33.D+, R34.2
- removed net N$56 (its old number): J41.D+, R42.2
- removed net N$57 (its old number): F6.2, J44.2, S11.1
- removed net N$6 (its old number): J2.D-, R3.2
- removed net RST: J4.1, R6.1, S3.1, U5.13
- removed net RST1: J14.1, R14.1, S4.1, U7.13
- removed net RST2: J22.1, R22.1, S6.1, U11.13
- removed net RST3: J30.1, R30.1, S8.1, U15.13
- removed net RST4: J38.1, R38.1, S10.1, U19.13
- removed net RST5: J46.1, R46.1, S12.1, U23.13
- new net !CS: U2.5, U3.41
- new net !CS1: U7.41, U8.5
- new net !CS2: U11.41, U12.5
- new net !CS3: U15.41, U16.5
- new net !CS4: U19.41, U20.5
- new net !CS5: U23.41, U24.5
- new net !RST: J10.5, J11.1, R6.1, S3.1, U3.13
- new net !RST1: J22.5, J23.1, R17.1, S4.1, U7.13
- new net !RST2: J34.5, J35.1, R28.1, S6.1, U11.13
- new net !RST3: J46.5, J47.1, R39.1, S8.1, U15.13
- new net !RST4: J58.5, J59.1, R50.1, S10.1, U19.13
- new net !RST5: J70.5, J71.1, R61.1, S12.1, U23.13
- new net N$2: D1.C, R7.2
- new net N$21: D8.A, R22.1
- new net N$3: D2.A, R3.1
- new net N$31: D9.C, R29.2
- new net N$32: D12.A, R33.1
- new net N$42: D15.C, R34.2
- new net N$43: D13.C, R40.2
- new net N$52: LED5.A, R48.1
- new net N$53: D19.C, R45.2
- new net N$61: R60.1, U21.5
- new net N$62: D22.C, R63.2
- new net N$63: LED6.A, R59.1
- new net N$64: D23.C, R56.2
- new net N$65: D21.C, R62.2
- new net N$66: D24.A, R66.1
- new net RFM_INT: U2.14, U3.1
- new net RFM_INT1: U7.1, U8.14
- new net RFM_INT2: U11.1, U12.14
- new net RFM_INT3: U15.1, U16.14
- new net RFM_INT4: U19.1, U20.14
- new net RFM_INT5: U23.1, U24.14
- new net RFM_IO1: JP1.1, U2.15
- new net RFM_IO10: JP10.1, U20.16
- new net RFM_IO11: JP11.1, U24.15
- new net RFM_IO12: JP12.1, U24.16
- new net RFM_IO2: JP2.1, U2.16
- new net RFM_IO3: JP3.1, U8.15
- new net RFM_IO4: JP4.1, U8.16
- new net RFM_IO5: JP5.1, U12.15
- new net RFM_IO6: JP6.1, U12.16
- new net RFM_IO7: JP7.1, U16.15
- new net RFM_IO8: JP8.1, U16.16
- new net RFM_IO9: JP9.1, U20.15
- new net RXLED: R10.1, U3.8
- new net RXLED1: R4.1, U7.8
- new net RXLED2: R23.1, U11.8
- new net RXLED3: R34.1, U15.8
- new net RXLED4: R45.1, U19.8
- new net RXLED5: R56.1, U23.8
- new net SCL: J2.4, U3.18
- new net SCL1: J21.4, U7.18
- new net SCL2: J33.4, U11.18
- new net SCL3: J45.4, U15.18
- new net SCL4: J57.4, U19.18
- new net SCL5: J69.4, U23.18
- new net SDA: J2.3, U3.19
- new net SDA1: J21.3, U7.19
- new net SDA2: J33.3, U11.19
- new net SDA3: J45.3, U15.19
- new net SDA4: J57.3, U19.19
- new net SDA5: J69.3, U23.19
- new net SHLD: J1.SHIELD, J1.SHIELD10, J1.SHIELD2, J1.SHIELD3, J1.SHIELD4, J1.SHIELD5, J1.SHIELD6, J1.SHIELD7, J1.SHIELD8, J1.SHIELD9
- new net SHLD1: J13.SHIELD, J13.SHIELD10, J13.SHIELD2, J13.SHIELD3, J13.SHIELD4, J13.SHIELD5, J13.SHIELD6, J13.SHIELD7, J13.SHIELD8, J13.SHIELD9
- new net SHLD2: J25.SHIELD, J25.SHIELD10, J25.SHIELD2, J25.SHIELD3, J25.SHIELD4, J25.SHIELD5, J25.SHIELD6, J25.SHIELD7, J25.SHIELD8, J25.SHIELD9
- new net SHLD3: J37.SHIELD, J37.SHIELD10, J37.SHIELD2, J37.SHIELD3, J37.SHIELD4, J37.SHIELD5, J37.SHIELD6, J37.SHIELD7, J37.SHIELD8, J37.SHIELD9
- new net SHLD4: J49.SHIELD, J49.SHIELD10, J49.SHIELD2, J49.SHIELD3, J49.SHIELD4, J49.SHIELD5, J49.SHIELD6, J49.SHIELD7, J49.SHIELD8, J49.SHIELD9
- new net SHLD5: J61.SHIELD, J61.SHIELD10, J61.SHIELD2, J61.SHIELD3, J61.SHIELD4, J61.SHIELD5, J61.SHIELD6, J61.SHIELD7, J61.SHIELD8, J61.SHIELD9
- new net STAT: R3.2, U3.32
- new net STAT1: R22.2, U7.32
- new net STAT2: R33.2, U11.32
- new net STAT3: R44.2, U15.32
- new net STAT4: R55.2, U19.32
- new net STAT5: R66.2, U23.32
- net 3.3V: now also C13.+, D1.A, D6.A, J10.2, J2.2, U3.14, U3.24, U3.34, U3.44; no longer C13.A, U5.14, U5.24, U5.34, U5.44
- net 3.3V1: now also C10.+, D3.A, D7.A, J17.2, J21.2, J22.2, R15.2, R17.2, U5.5, U8.13; no longer C10.A, J13.2, R14.2, R4.2, U4.13, U8.5
- net 3.3V2: now also C24.+, D11.A, D9.A, J29.2, J33.2, J34.2, R26.2, R28.2, U10.5, U12.13; no longer C24.A, J21.2, R20.2, R22.2, U10.13, U12.5
- net 3.3V3: now also C34.+, D13.A, D15.A, J41.2, J45.2, J46.2, R37.2, R39.2, U14.5, U16.13; no longer C34.A, J29.2, R28.2, R30.2, U14.13, U16.5
- net 3.3V4: now also C44.+, D17.A, D19.A, J53.2, J57.2, J58.2, R48.2, R50.2, U18.5, U20.13; no longer C44.A, J37.2, R36.2, R38.2, U18.13, U20.5
- net 3.3V5: now also C54.+, D21.A, D23.A, J65.2, J69.2, J70.2, R59.2, R61.2, U22.5, U24.13; no longer C54.A, J45.2, R44.2, R46.2, U22.13, U24.5
- net A0: now also J11.6, U3.36; no longer J4.6, U5.36
- net A1: now also J11.5, U3.37; no longer J4.5, U5.37
- net A10: now also J35.6, U11.36; no longer J14.2, U7.40
- net A11: now also J35.5, U11.37; no longer U7.41
- net A12: now also J35.4, U11.38; no longer J22.6, U11.36
- net A13: now also J35.3, U11.39; no longer J22.5, U11.37
- net A14: now also J35.2, U11.40; no longer J22.4, U11.38
- net A15: now also J47.6, U15.36; no longer J22.3, U11.39
- net A16: now also J47.5, U15.37; no longer J22.2, U11.40
- net A17: now also J47.4, U15.38; no longer U11.41
- net A18: now also J47.3, U15.39; no longer J30.6, U15.36
- net A19: now also J47.2, U15.40; no longer J30.5, U15.37
- net A2: now also J11.4, U3.38; no longer J4.4, U5.38
- net A20: now also J59.6, U19.36; no longer J30.4, U15.38
- net A21: now also J59.5, U19.37; no longer J30.3, U15.39
- net A22: now also J59.4, U19.38; no longer J30.2, U15.40
- net A23: now also J59.3, U19.39; no longer U15.41
- net A24: now also J59.2, U19.40; no longer J38.6, U19.36
- net A25: now also J71.6, U23.36; no longer J38.5, U19.37
- net A26: now also J71.5, U23.37; no longer J38.4, U19.38
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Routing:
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- added copper zone on layer 1, net SHLD
- added copper zone on layer 16, net SHLD
- added copper zone on layer 1, net SHLD1
- added copper zone on layer 16, net SHLD1
- added copper zone on layer 1, net SHLD2
- added copper zone on layer 16, net SHLD2
- added copper zone on layer 1, net SHLD3
- added copper zone on layer 16, net SHLD3
- added copper zone on layer 1, net SHLD4
- added copper zone on layer 16, net SHLD4
- added copper zone on layer 1, net SHLD5
- added copper zone on layer 16, net SHLD5
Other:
- board size 101.9 x 104.9 mm -> 105.7 x 98.6 mm
- board text added: "+"
- board text added: "-"
- board text added: "RFM69 or RFM95W"
- board text added: "Route Out"
- board text added: "x02"
- board text removed: "x01"
